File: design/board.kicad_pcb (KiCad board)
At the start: 2 copper layers, 96.5 x 81.3 mm, 14 parts, among them J1 Mic, J2 DEBUG_CONN, J3 PWR_CONN, J4 0.97" OLED, J5 WS2812b, SW1 SW_Push, U1 NodeMCU1.0(ESP-12E), U2 BME280

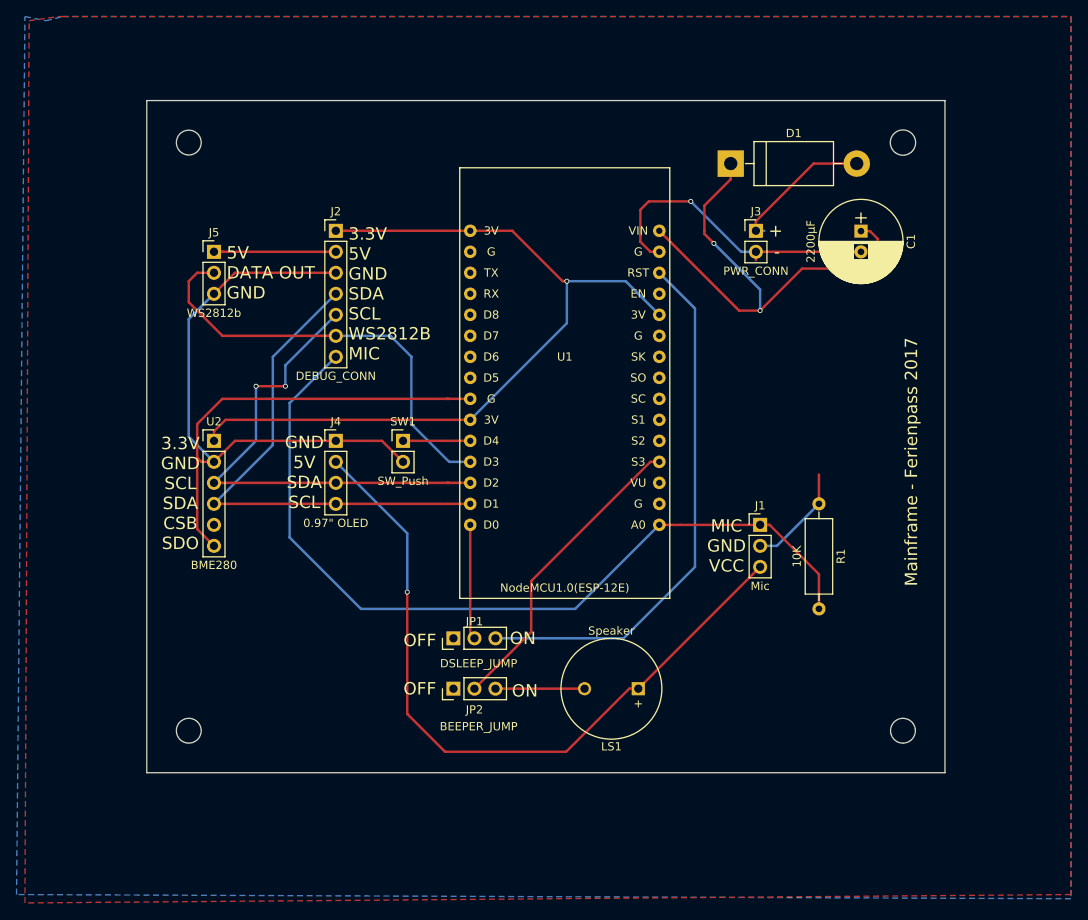
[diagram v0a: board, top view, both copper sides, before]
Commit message: improved PCB-Layout for next Year
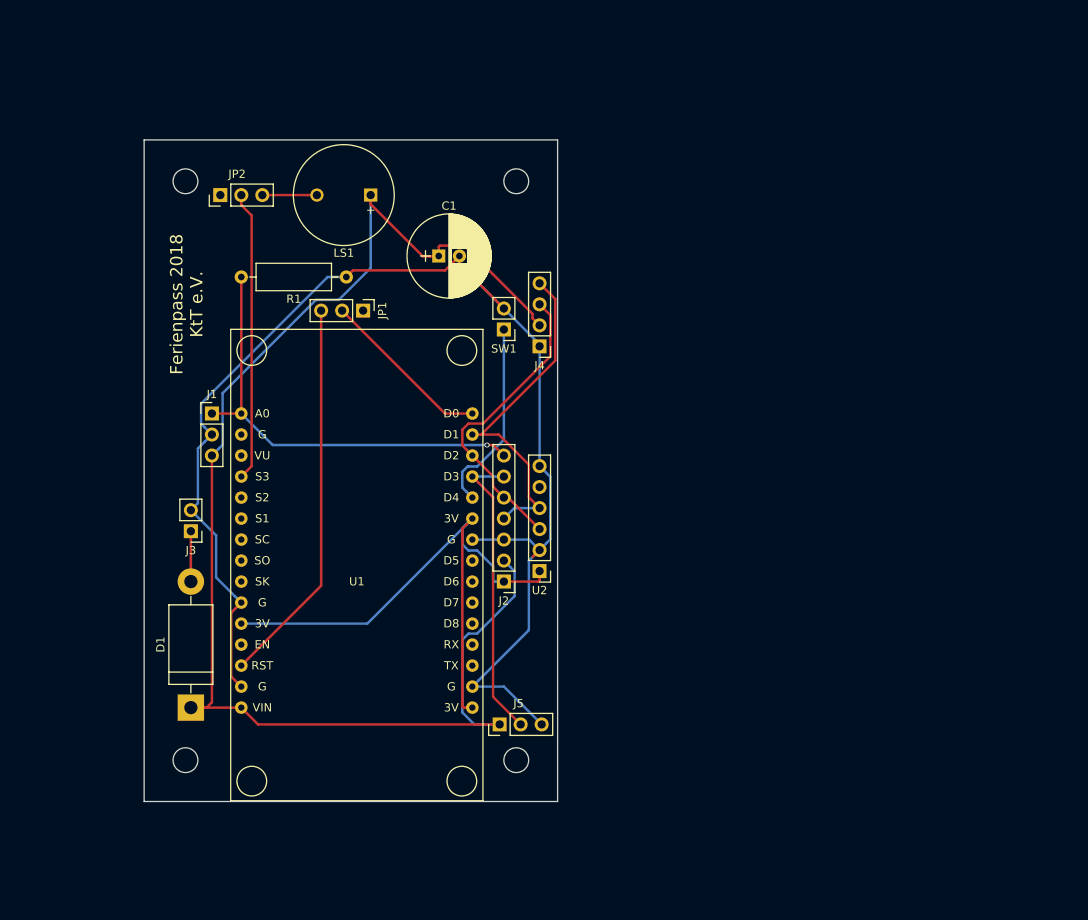
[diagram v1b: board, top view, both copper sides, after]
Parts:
- SW1: footprint Pin_Headers:Pin_Header_Straight_1x02_Pitch2.54mm -> Socket_Strips:Socket_Strip_Straight_1x02_Pitch2.54mm
- moved D1 92.7 mm to (25.7, 88.6), turned to 90 degrees
- moved J3 77.4 mm to (25.7, 67.3), turned to 180 degrees
- moved LS1 67.9 mm to (47.4, 26.7)
- moved J1 67.6 mm to (28.2, 53.1)
- moved J5 66.8 mm to (63.0, 90.7), turned to 90 degrees
- moved JP2 66.0 mm to (29.2, 26.7)
- moved R1 63.4 mm to (44.5, 36.6), turned to 180 degrees
- moved C1 51.1 mm to (55.6, 34.0), turned to 0 degrees
- moved J2 47.0 mm to (63.5, 73.4), turned to 180 degrees
- moved U2 42.4 mm to (67.8, 72.1), turned to 180 degrees
- moved JP1 41.1 mm to (46.5, 40.6), turned to 270 degrees
- moved U1 37.0 mm to (45.7, 73.4), turned to 0 degrees
- moved J4 27.2 mm to (67.8, 45.0), turned to 180 degrees
- moved SW1 18.2 mm to (63.5, 42.9), turned to 180 degrees
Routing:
- net MIC: track 102.6 -> 53.9 mm, vias 0 -> 1
- net +3V3: track 97.6 -> 74.7 mm, vias 1 -> 0
- net SCL: track 59.7 -> 37.3 mm, vias 2 -> 0
- net SDA: track 62.5 -> 41.8 mm
- net Net-(JP1-Pad3): track 65.1 -> 46.9 mm
- net WS2812b: track 52.8 -> 36.2 mm
- net Net-(SW1-Pad1): track 8.13 -> 23.6 mm
- net Net-(D1-Pad2): track 17.2 -> 6.10 mm
- net D0: track 13.9 -> 20.9 mm
- net VCC: track 163.4 -> 168.7 mm, vias 3 -> 0
- net Net-(JP2-Pad3): track 10.8 -> 6.60 mm
- net SD3: track 37.3 -> 35.1 mm
- net GND: track 166.1 -> 164.0 mm, vias 1 -> 0
- removed copper zone on F.Cu, net GND
- removed copper zone on B.Cu, net VCC
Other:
- board size 96.5 x 81.3 mm -> 50 x 80 mm
- board text added: "Ferienpass 2018 KtT e.V."
- board text removed: "+"
- board text removed: "-"
- board text removed: "3.3V 5V GND SDA SCL WS2812B MIC"
- board text removed: "3.3V GND SCL SDA CSB SDO"
- board text removed: "5V DATA OUT GND"
- board text removed: "GND 5V SDA SCL"
- board text removed: "MIC GND VCC"
- board text removed: "Mainframe - Ferienpass 2017"
- board text removed: "OFF"
- board text removed: "ON"
